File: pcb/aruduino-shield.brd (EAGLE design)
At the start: 68.6 x 61.9 mm, 23 parts, among them J1 POWER_JACKPOWER_JACK_SLOT

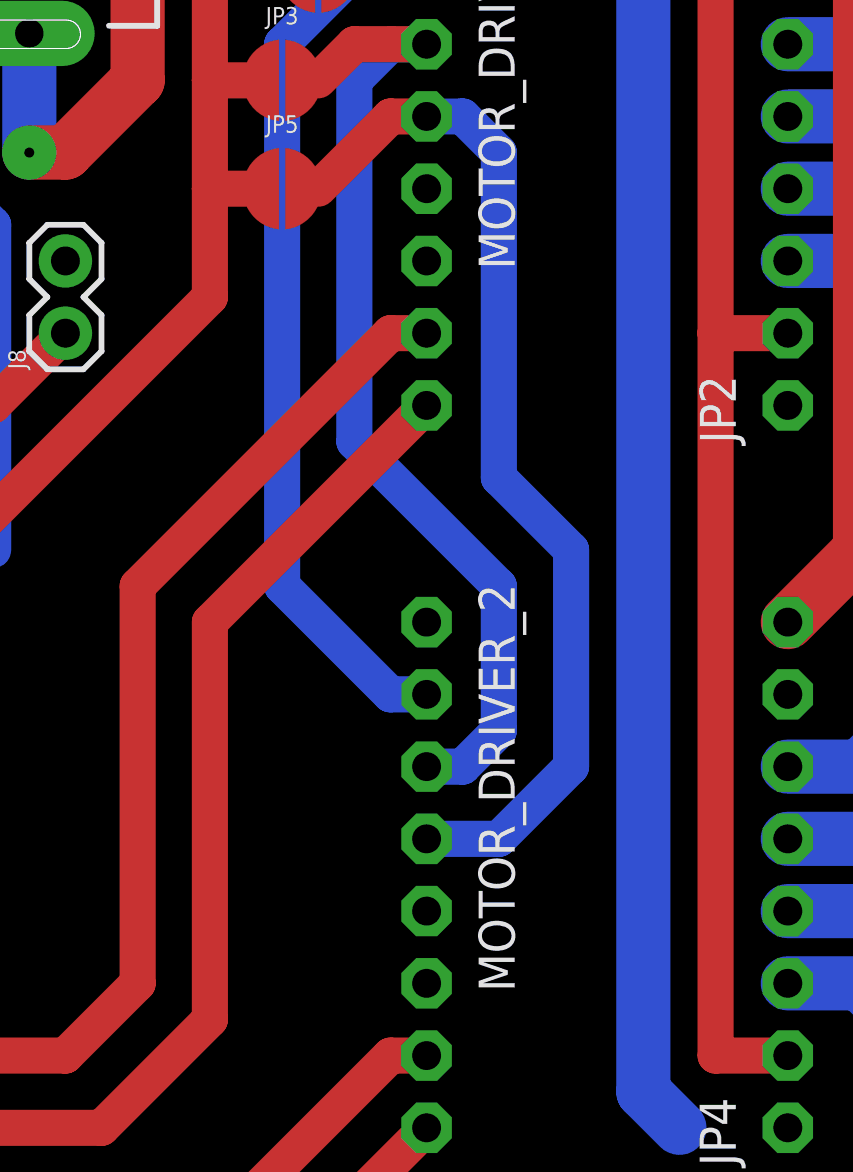
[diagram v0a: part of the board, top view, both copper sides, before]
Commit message: small fixes
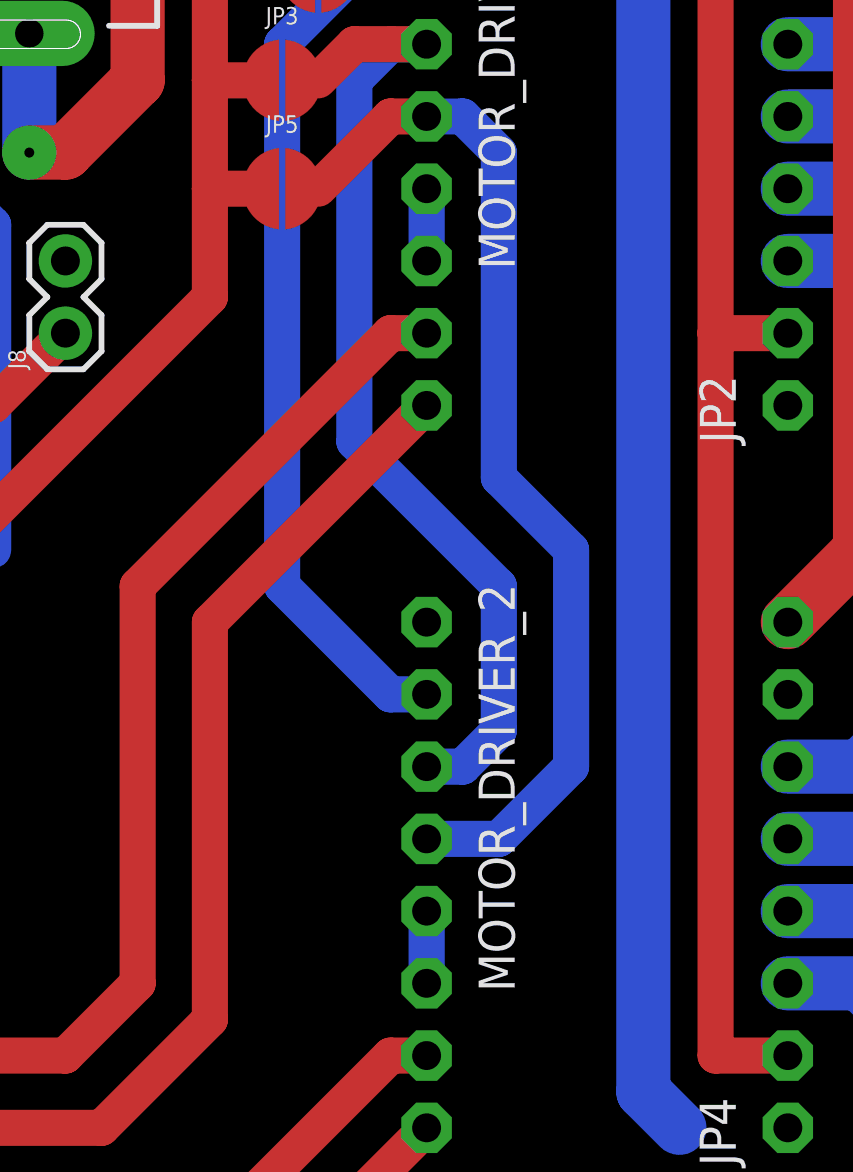
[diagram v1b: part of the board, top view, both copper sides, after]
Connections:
- net DIR_1: now also B1.A5, MOTOR_DRIVER_2.8; no longer B1.A3, MOTOR_DRIVER_1.8
- net DIR_2: now also B1.A3, MOTOR_DRIVER_1.8; no longer B1.A5, MOTOR_DRIVER_2.8
- net FWD_1: now also B1.D3, J9.1; no longer B1.D5, J12.1
- net FWD_2: now also B1.D5, J12.1; no longer B1.D3, J9.1
- net REED_SWITCH_1: now also B1.D12, J4.1; no longer B1.D13, J11.1
- net REED_SWITCH_2: now also B1.D13, J11.1; no longer B1.D12, J4.1
- net REV_1: now also B1.D2, J10.1; no longer B1.D4, J13.1
- net REV_2: now also B1.D4, J13.1; no longer B1.D2, J10.1
- net STEP_1: now also B1.A4, MOTOR_DRIVER_2.7; no longer B1.A2, MOTOR_DRIVER_1.7
- net STEP_2: now also B1.A2, MOTOR_DRIVER_1.7; no longer B1.A4, MOTOR_DRIVER_2.7
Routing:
- net STEP_2: track 22.4 -> 39.0 mm
- net STEP_1: track 39.0 -> 22.4 mm
- net DIR_2: track 22.4 -> 39.0 mm
- net DIR_1: track 39.0 -> 22.4 mm
- net REV_2: track 15.9 -> 12.7 mm
- net REV_1: track 12.7 -> 15.9 mm
- net REED_SWITCH_2: track 16.8 -> 19.9 mm
- net REED_SWITCH_1: track 19.9 -> 16.8 mm
- net N$2: track 0.00 -> 2.54 mm
- net N$1: track 0.00 -> 2.54 mm
- net FWD_2: track 14.8 -> 13.8 mm
- net FWD_1: track 13.8 -> 14.8 mm
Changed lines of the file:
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@@
 <?xml version="1.0" encoding="utf-8"?>
 <!DOCTYPE eagle SYSTEM "eagle.dtd">
-<eagle version="9.6.0">
+<eagle version="9.6.2">
 <drawing>
 <settings>
@@
 <via x="6.35" y="31.75" extent="1-16" drill="0.35" diameter="1.905"/>
 </signal>
-<signal name="STEP_2">
+<signal name="STEP_1">
 <contactref element="MOTOR_DRIVER_2" pad="7"/>
 <wire x1="24.13" y1="13.97" x2="22.86" y2="13.97" width="1.27" layer="1"/>
@@
 <wire x1="17.78" y1="8.89" x2="3.81" y2="8.89" width="1.27" layer="1"/>
 </signal>
-<signal name="DIR_2">
+<signal name="DIR_1">
 <contactref element="MOTOR_DRIVER_2" pad="8"/>
 <wire x1="24.13" y1="11.43" x2="19.05" y2="6.35" width="1.27" layer="1"/>
@@
 <wire x1="44.45" y1="14.9" x2="40.98" y2="14.9" width="1.905" layer="16"/>
 </signal>
-<signal name="STEP_1">
+<signal name="STEP_2">
 <contactref element="MOTOR_DRIVER_1" pad="7"/>
 <wire x1="24.13" y1="39.37" x2="22.86" y2="39.37" width="1.27" layer="1"/>
@@
 <wire x1="11.43" y1="13.97" x2="3.81" y2="13.97" width="1.27" layer="1"/>
 </signal>
-<signal name="DIR_1">
+<signal name="DIR_2">
 <contactref element="MOTOR_DRIVER_1" pad="8"/>
 <wire x1="24.13" y1="36.83" x2="16.51" y2="29.21" width="1.27" layer="1"/>
@@
 <wire x1="8.89" y1="36.83" x2="3.81" y2="36.83" width="1.27" layer="1"/>
 </signal>
-<signal name="FWD_1">
+<signal name="FWD_2">
 <wire x1="60.96" y1="19.05" x2="63.5" y2="21.59" width="1.27" layer="1"/>
 <contactref element="B1" pad="D5"/>
@@
 <wire x1="64.77" y1="21.59" x2="63.5" y2="21.59" width="1.27" layer="1"/>
 </signal>
-<signal name="REV_1">
+<signal name="REV_2">
 <contactref element="B1" pad="D4"/>
 <contactref element="J13" pad="1"/>
 <wire x1="64.77" y1="16.51" x2="52.07" y2="16.51" width="1.27" layer="1"/>
 </signal>
-<signal name="FWD_2">
+<signal name="FWD_1">
 <wire x1="55.88" y1="13.97" x2="60.96" y2="8.89" width="1.27" layer="1"/>
 <contactref element="B1" pad="D3"/>
@@
 <wire x1="64.77" y1="8.89" x2="60.96" y2="8.89" width="1.27" layer="1"/>
 </signal>
-<signal name="REV_2">
+<signal name="REV_1">
 <wire x1="54.61" y1="11.43" x2="62.23" y2="3.81" width="1.27" layer="1"/>
 <contactref element="B1" pad="D2"/>
@@
 <wire x1="52.07" y1="28.194" x2="54.61" y2="28.194" width="1.27" layer="1"/>
 </signal>
-<signal name="REED_SWITCH_1">
+<signal name="REED_SWITCH_2">
 <contactref element="J11" pad="1"/>
 <contactref element="B1" pad="D13"/>
@@
 <wire x1="62.23" y1="49.53" x2="62.23" y2="52.07" width="1.27" layer="1"/>
 </signal>
-<signal name="REED_SWITCH_2">
+<signal name="REED_SWITCH_1">
 <contactref element="J4" pad="1"/>
 <contactref element="B1" pad="D12"/>
@@
 <contactref element="MOTOR_DRIVER_2" pad="6"/>
 <contactref element="MOTOR_DRIVER_2" pad="5"/>
-<wire x1="24.13" y1="16.51" x2="24.13" y2="19.05" width="0" layer="19" extent="1-1"/>
+<wire x1="24.13" y1="16.51" x2="24.13" y2="19.05" width="1.27" layer="16"/>
 </signal>
 <signal name="N$2">
 <contactref element="MOTOR_DRIVER_1" pad="6"/>
 <contactref element="MOTOR_DRIVER_1" pad="5"/>
-<wire x1="24.13" y1="41.91" x2="24.13" y2="44.45" width="0" layer="19" extent="1-1"/>
+<wire x1="24.13" y1="41.91" x2="24.13" y2="44.45" width="1.27" layer="16"/>
 </signal>
 <signal name="GND_TOP">
